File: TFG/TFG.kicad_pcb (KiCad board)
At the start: 2 copper layers, 68.3 x 67.9 mm, 36 parts, among them IC1 MC74VHC1GT04DFT2G, IC2 TS1117BCW50 RPG, IC3 TS1117BCW50 RPG, J1 Jack-DC, J2 CON-SMA-EDGE-SRP, J3 CON-SMA-EDGE-SRP, Q1 BFP420

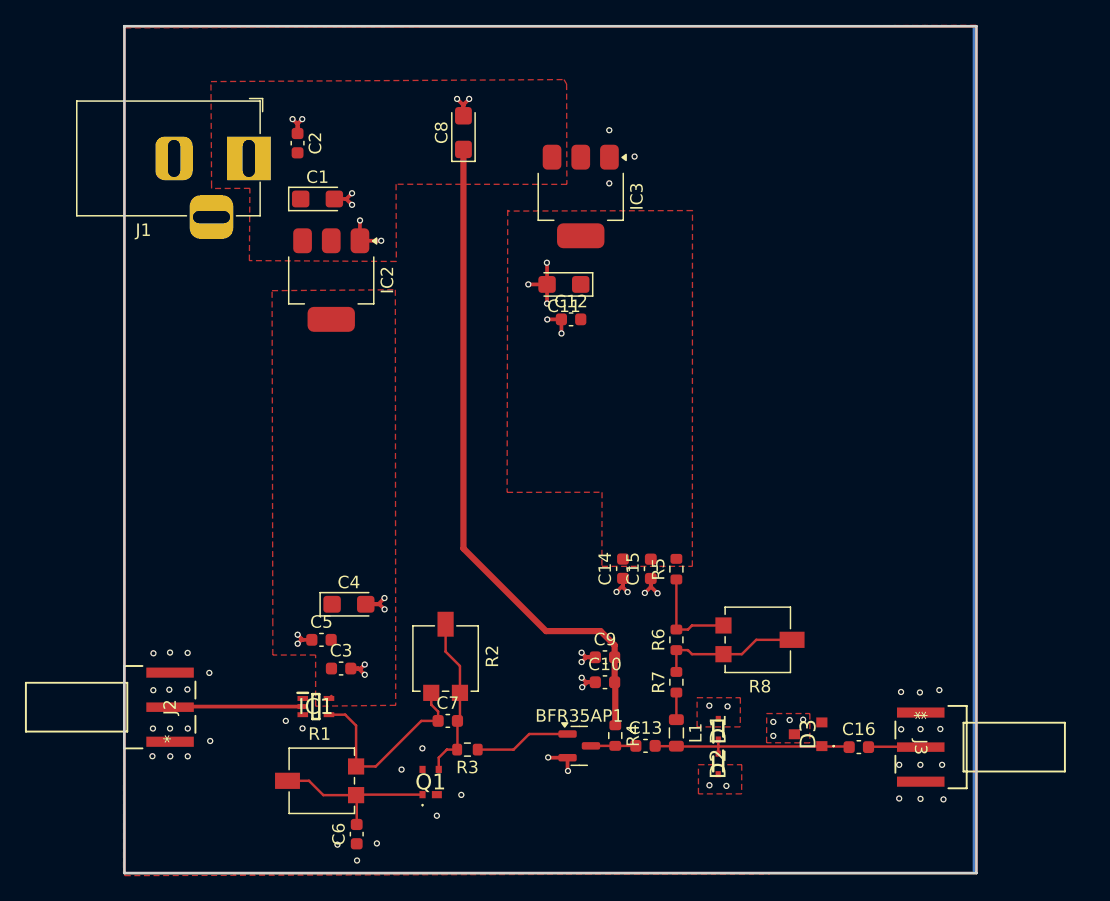
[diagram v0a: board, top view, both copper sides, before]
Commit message: Final design for Ultrawideband pulse generator PCB - v1
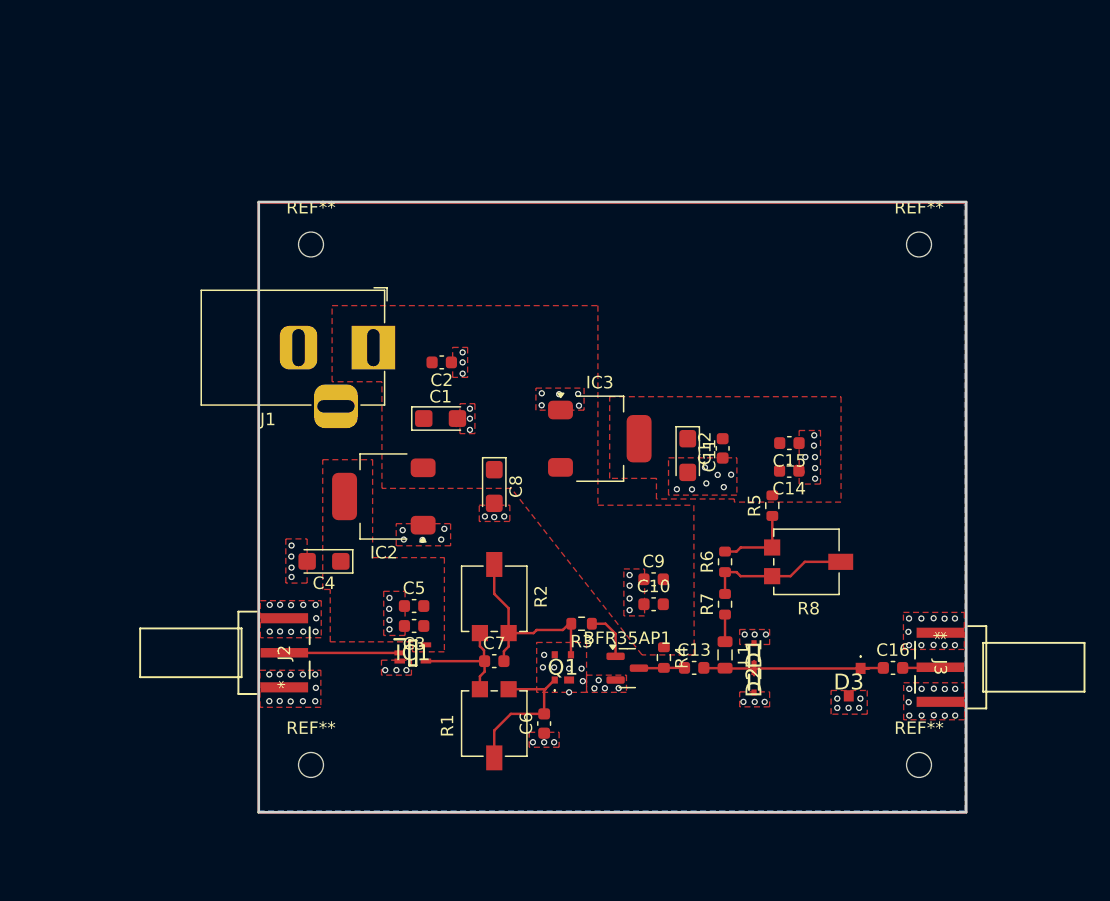
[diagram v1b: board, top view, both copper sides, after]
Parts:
- added REF**: MountingHole_2mm, MountingHole:MountingHole_2mm, F.Cu at (50.9, 75.8)
- added REF**: MountingHole_2mm, MountingHole:MountingHole_2mm, F.Cu at (50.9, 34.1)
- added REF**: MountingHole_2mm, MountingHole:MountingHole_2mm, F.Cu at (99.6, 34.1)
- added REF**: MountingHole_2mm, MountingHole:MountingHole_2mm, F.Cu at (99.6, 75.8)
- moved C8 28.5 mm to (65.5, 53.5), turned to -90 degrees
- moved C2 21.0 mm to (61.3, 43.6), turned to 180 degrees
- moved C1 20.2 mm to (61.2, 48.1)
- moved IC3 19.5 mm to (74.0, 49.7), turned to 0 degrees
- moved J1 18.2 mm to (55.9, 42.4)
- moved IC2 17.9 mm to (56.7, 54.3), turned to 180 degrees
- moved C6 17.4 mm to (69.5, 72.5)
- moved C11 16.9 mm to (81.1, 51.0), turned to -90 degrees
- moved C12 16.0 mm to (83.9, 50.5), turned to 90 degrees
- moved C14 15.5 mm to (89.2, 52.2), turned to 180 degrees
- moved C15 15.0 mm to (89.2, 50.0), turned to 180 degrees
- moved R1 14.6 mm to (65.5, 72.5), turned to 90 degrees
- moved Q1 14.0 mm to (71.0, 68.0)
- moved R3 13.6 mm to (72.5, 64.5)
- moved J2 10.1 mm to (47.9, 66.8)
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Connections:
- J1 pad 3: (no net) -> GND
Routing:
- net /V12v: track 54.0 -> 0.57 mm
- net GND: track 37.7 -> 0.32 mm, vias 75 -> 116
- net Net-(IC1-Y): track 16.4 -> 9.75 mm
- net Net-(BFR35AP1-B): track 7.57 -> 4.04 mm
- net Net-(Q1-C): track 13.5 -> 16.2 mm
- net /Vout: track 5.46 -> 3.08 mm
- net Net-(R5-Pad1): track 7.95 -> 6.44 mm
- net /V3v_in: track 10.5 -> 9.27 mm
- net /V5v: track 1.05 -> 0.00 mm
- net Net-(Q1-B): track 13.7 -> 12.8 mm
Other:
- board size 68.3 x 67.9 mm -> 56.7 x 48.9 mm
